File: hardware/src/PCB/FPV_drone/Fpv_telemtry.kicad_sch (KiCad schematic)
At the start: 9 parts, among them IC6 INA186A1IDCKR, IC9 W25Q128JVPIQ, U1 SPA06-003, U3 ICM-42688-P, U4 ICM-42688-P

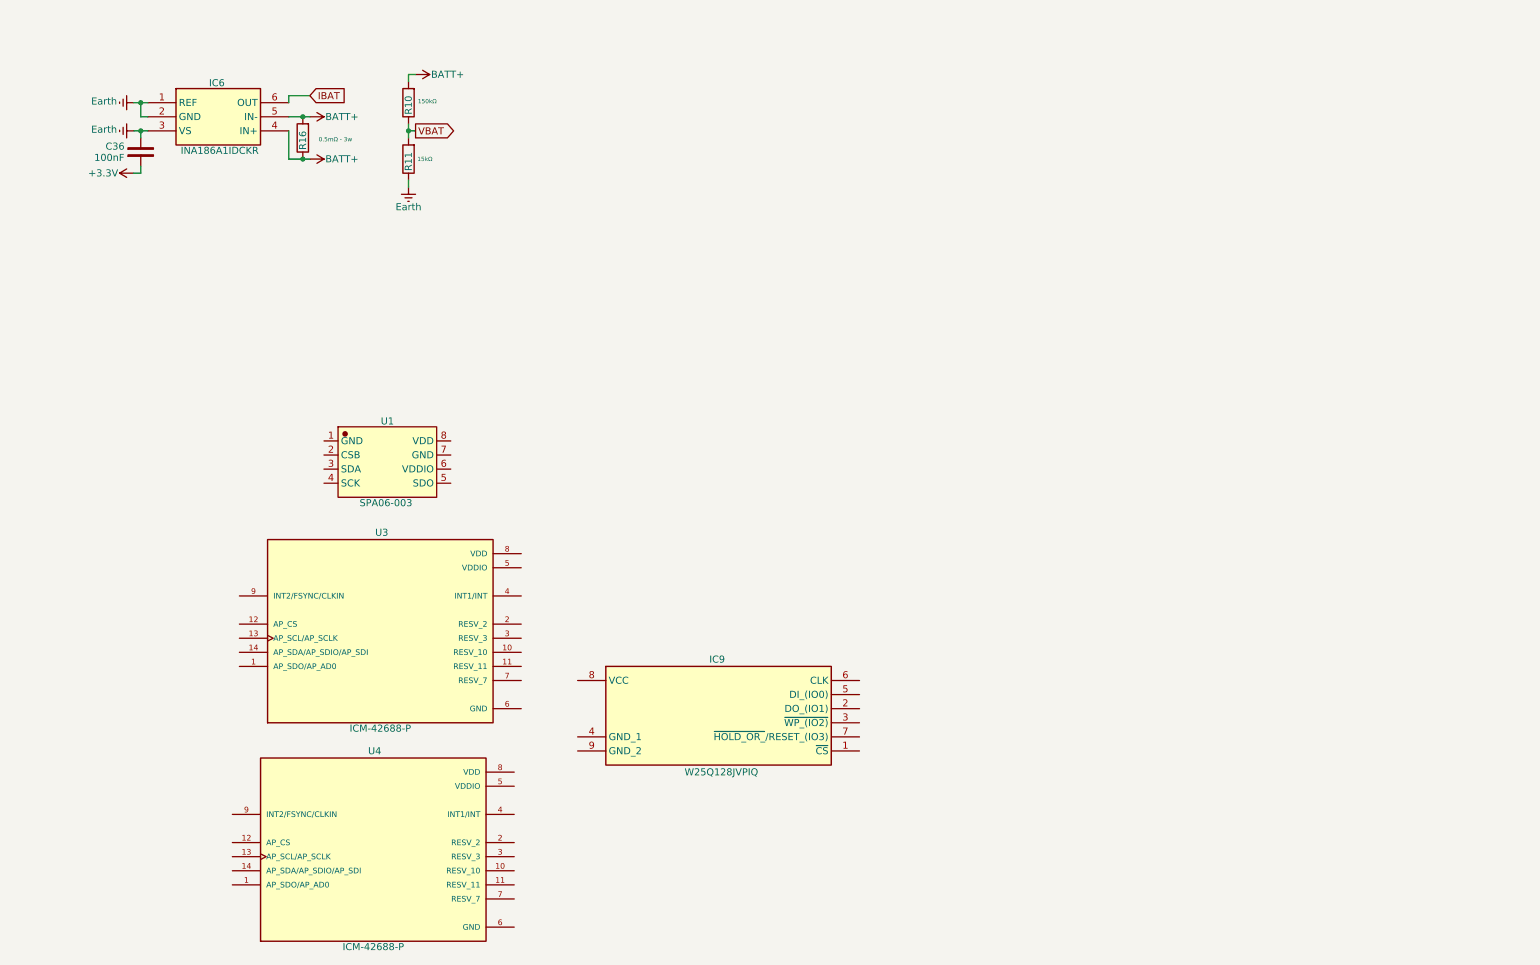
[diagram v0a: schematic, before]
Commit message: Update: schem almost finish
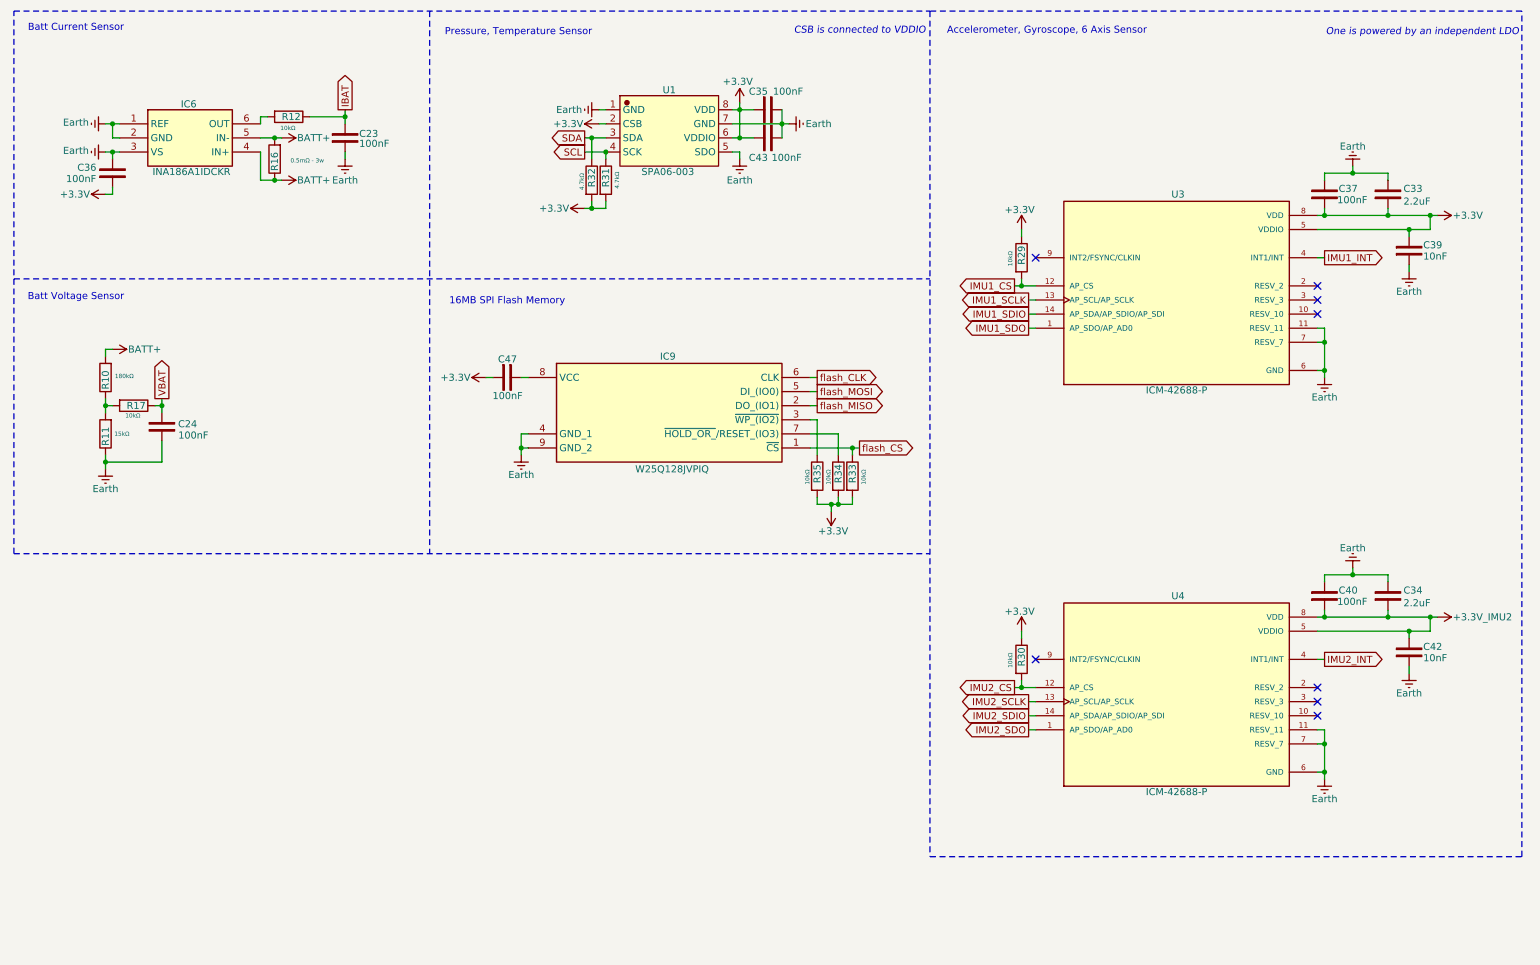
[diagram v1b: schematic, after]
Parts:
- added C23, C24, C35, C37, C40, C43, C47: 100nF, Capacitor_THT:C_Disc_D3.0mm_W2.0mm_P2.50mm, symbol PCM_SL_Devices:Capacitor_NP
- added C33, C34: 2.2uF, Capacitor_THT:C_Disc_D3.0mm_W2.0mm_P2.50mm, symbol PCM_SL_Devices:Capacitor_NP
- added C39, C42: 10nF, Capacitor_THT:C_Disc_D3.0mm_W2.0mm_P2.50mm, symbol PCM_SL_Devices:Capacitor_NP
- added R12, R17, R29, R30, R33, R34, R35: 10kΩ, symbol Device:R
- added R31, R32: 4.7kΩ, symbol Device:R
- R10: value 150kΩ -> 180kΩ
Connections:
- net +3.3V: now also U1.2 (CSB), U1.6 (VDDIO), U1.8 (VDD), U3.5 (VDDIO), U3.8 (VDD), C33.1, C35.1, C37.1, C39.2, C43.1, C47.1, R29.1, R30.1, R31.2, R32.2, R33.2, R34.2, R35.2
- net Earth: now also IC9.4 (GND_1), IC9.9 (GND_2), U1.1 (GND), U1.5 (SDO), U1.7 (GND), U3.11 (RESV_11), U3.6 (GND), U3.7 (RESV_7), U4.11 (RESV_11), U4.6 (GND), U4.7 (RESV_7), C23.1, C24.2, C33.2, C34.2, C35.2, C37.2, C39.1, C40.2, C42.1, C43.2
- net IBAT: now also C23.2, R12.1; no longer IC6.6 (OUT)
- net VBAT: now also C24.1, R17.1; no longer R10.1, R11.2
- net IMU1_SDO: now reaches U3.1 (AP_SDO/AP_AD0)
- net IMU1_CS: now reaches U3.12 (AP_CS)
- net IMU1_CS: now also R29.2
- net IMU1_SCLK: now reaches U3.13 (AP_SCL/AP_SCLK)
- net IMU1_SDIO: now reaches U3.14 (AP_SDA/AP_SDIO/AP_SDI)
- net IMU1_INT: now reaches U3.4 (INT1/INT)
- net IMU2_SDO: now reaches U4.1 (AP_SDO/AP_AD0)
- net IMU2_CS: now reaches U4.12 (AP_CS)
- net IMU2_CS: now also R30.2
- net IMU2_SCLK: now reaches U4.13 (AP_SCL/AP_SCLK)
- net IMU2_SDIO: now reaches U4.14 (AP_SDA/AP_SDIO/AP_SDI)
- net IMU2_INT: now reaches U4.4 (INT1/INT)
- net +3.3V_IMU2: now reaches U4.5 (VDDIO)
- net +3.3V_IMU2: now also U4.8 (VDD), C34.1, C40.1, C42.2
- net SDA: now reaches U1.3 (SDA)
- net SDA: now also R32.1
- net SCL: now reaches U1.4 (SCK)
- net SCL: now also R31.1
- net flash_CS: now reaches IC9.1 (~{CS})
- net flash_CS: now also R33.1
- net flash_MISO: now reaches IC9.2 (DO_(IO1))
- net at IC9.3 (~{WP_(IO2)}): now also R35.1
- net flash_MOSI: now reaches IC9.5 (DI_(IO0))
- net flash_CLK: now reaches IC9.6 (CLK)
- net at IC9.7 (~{HOLD_OR_}/RESET_(IO3)): now also R34.1
- net at IC9.8 (VCC): now also C47.2
- new net: R10.1, R11.2, R17.2
- new net: IC6.6 (OUT), R12.2
- no-connect marks 0 -> 8
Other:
- note added: "16MB SPI Flash Memory"
- note added: "Accelerometer, Gyroscope, 6 Axis Sensor"
- note added: "Batt Current Sensor"
- note added: "Batt Voltage Sensor"
- note added: "CSB is connected to VDDIO"
- note added: "One is powered by an independent LDO"
- note added: "Pressure, Temperature Sensor"
- moved on the sheet: C36, IC6, IC9, R10, R11, R16, U1, U3, U4
